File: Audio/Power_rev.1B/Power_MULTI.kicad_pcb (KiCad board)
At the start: 2 copper layers, 175.3 x 76.2 mm, 76 parts, among them P1 CONN_01X02, P2 CONN_01X02, P3 CONN_01X02, P4 CONN_01X02, Q1 NPN(TO-220-BCE), Q2 PNP(TO-220-BCE), Q3 NPN(TO-220-BCE), Q4 PNP(TO-220-BCE)

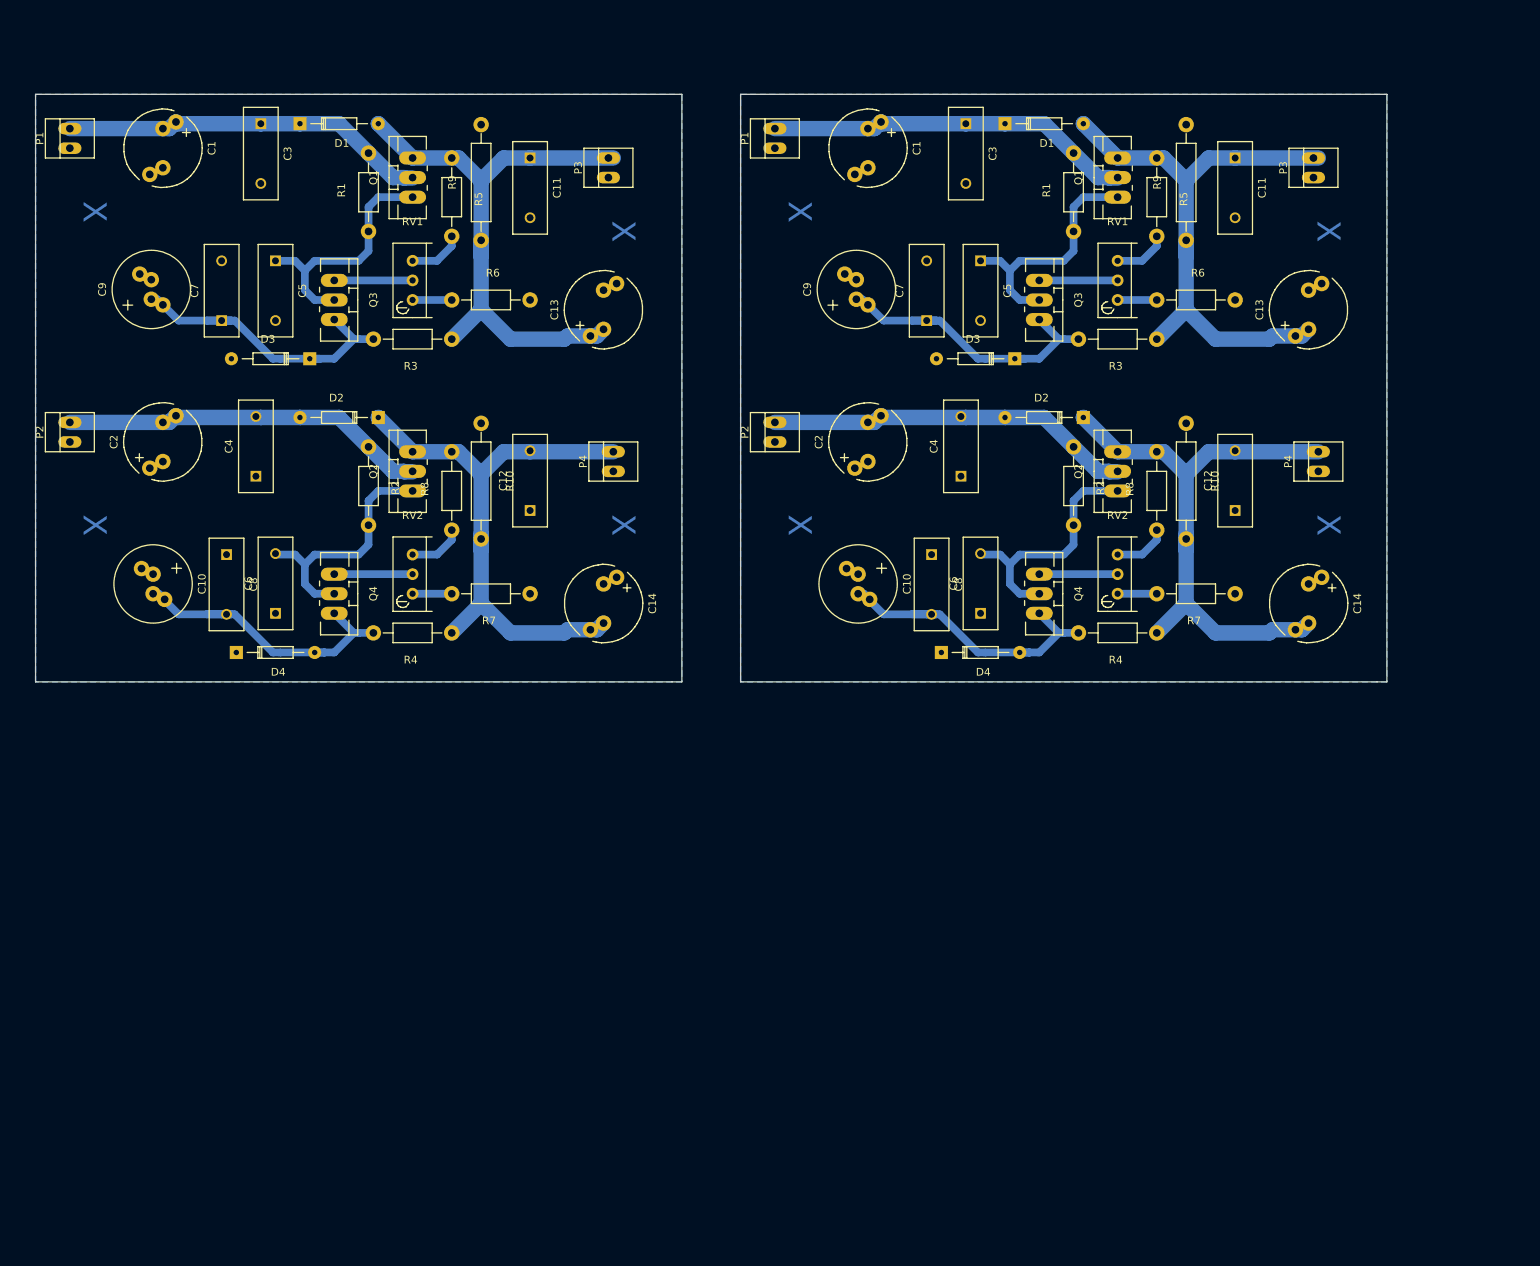
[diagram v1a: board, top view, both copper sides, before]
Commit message: Fixes
More fixes done
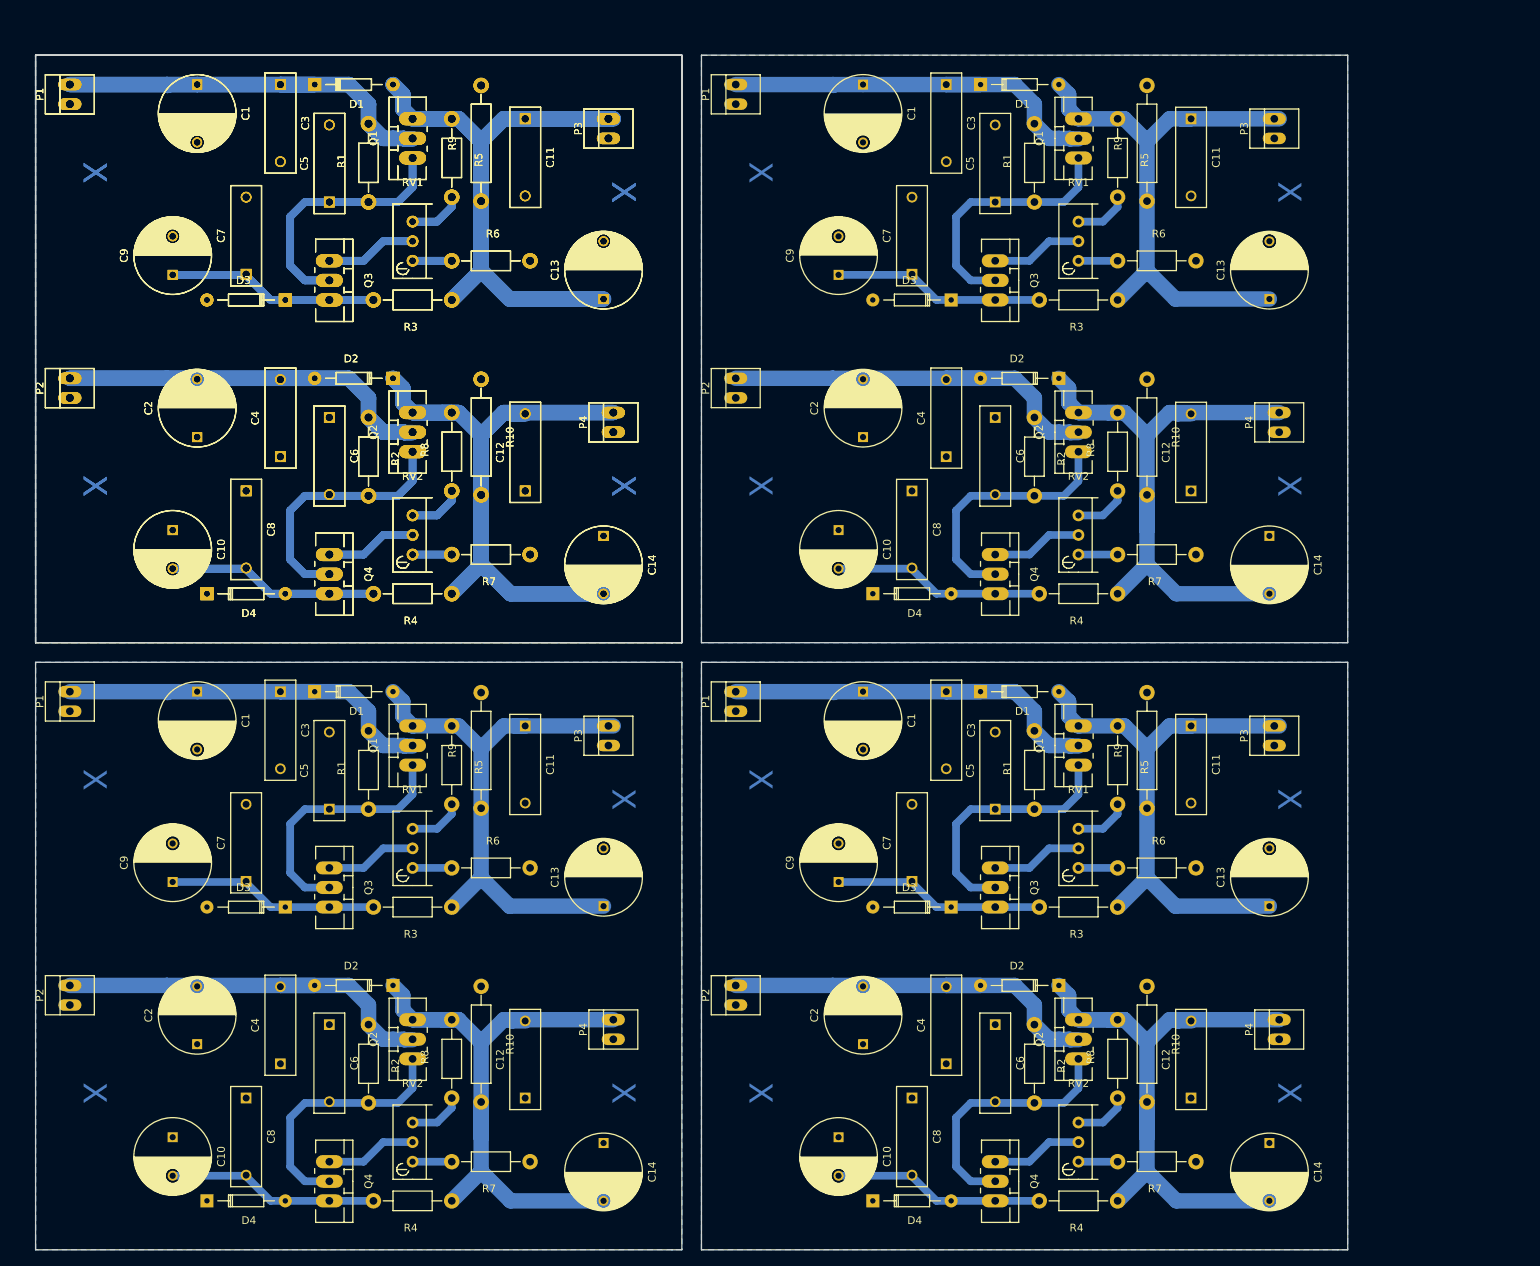
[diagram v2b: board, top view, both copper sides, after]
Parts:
- removed the C1 at (41.9, 37.5)
- removed the C1 at (133.3, 37.5)
- removed the C10 at (40.6, 94.0)
- removed the C10 at (132.1, 94.0)
- removed the C11 at (89.5, 38.7)
- removed the C11 at (181.0, 38.7)
- removed the C12 at (89.5, 84.5)
- removed the C12 at (181.0, 84.5)
- removed the C13 at (99.1, 58.4)
- removed the C13 at (190.5, 58.4)
- removed the C14 at (99.1, 96.5)
- removed the C14 at (190.5, 96.5)
- removed the C2 at (41.9, 75.6)
- removed the C2 at (133.3, 75.6)
- removed the C3 at (54.6, 34.3)
- removed the C3 at (146.1, 34.3)
- removed the C4 at (54.0, 80.0)
- removed the C4 at (145.4, 80.0)
- removed the C5 at (56.5, 52.1)
- removed the C5 at (148.0, 52.1)
- removed the C6 at (56.5, 97.8)
- removed the C6 at (148.0, 97.8)
- removed the C7 at (49.5, 59.8)
- removed the C7 at (141.0, 59.8)
- removed the C8 at (50.2, 90.2)
- removed the C8 at (141.6, 90.2)
- removed the C9 at (40.4, 55.8)
- removed the C9 at (131.8, 55.8)
- removed the D1 at (59.7, 34.3)
- removed the D1 at (151.1, 34.3)
- removed the D2 at (69.8, 72.4)
- removed the D2 at (161.3, 72.4)
- removed the D3 at (61.0, 64.8)
- removed the D3 at (152.4, 64.8)
- removed the D4 at (51.4, 102.9)
- removed the D4 at (142.9, 102.9)
- removed the P1 at (29.8, 36.2)
- removed the P1 at (121.3, 36.2)
- removed the P2 at (29.8, 74.3)
- removed the P2 at (121.3, 74.3)
- removed the P3 at (99.7, 40.0)
- removed the P3 at (191.1, 40.0)
- removed the P4 at (100.3, 78.1)
- removed the P4 at (191.8, 78.1)
- removed the Q1 at (74.3, 41.3)
- removed the Q1 at (165.7, 41.3)
- removed the Q2 at (74.3, 79.4)
- removed the Q2 at (165.7, 79.4)
- removed the Q3 at (64.1, 57.1)
- removed the Q3 at (155.6, 57.1)
- removed the Q4 at (64.1, 95.2)
- removed the Q4 at (155.6, 95.2)
- removed the R1 at (68.6, 43.2)
- removed the R1 at (160.0, 43.2)
- removed the R10 at (83.2, 80.6)
- removed the R10 at (174.6, 80.6)
- removed the R2 at (68.6, 81.3)
- removed the R2 at (160.0, 81.3)
- removed the R3 at (74.3, 62.2)
- removed the R3 at (165.7, 62.2)
- removed the R4 at (74.3, 100.3)
- removed the R4 at (165.7, 100.3)
- removed the R5 at (79.4, 43.8)
- removed the R5 at (170.8, 43.8)
- removed the R6 at (84.5, 57.1)
- removed the R6 at (175.9, 57.1)
- removed the R7 at (84.5, 95.2)
- removed the R7 at (175.9, 95.2)
- removed the R8 at (79.4, 81.9)
- removed the R8 at (170.8, 81.9)
- removed the R9 at (83.2, 41.9)
- removed the R9 at (174.6, 41.9)
- removed the RV1 at (74.3, 57.1)
- removed the RV1 at (165.7, 57.1)
- removed the RV2 at (74.3, 95.2)
- removed the RV2 at (165.7, 95.2)
- added C1 (x2): 820uF,100V, Capacitors_ThroughHole:C_Radial_D10_L20_P7.5, F.Cu at (46.4, 29.2)
- added C1: 820uF,100V, Capacitors_ThroughHole:C_Radial_D10_L20_P7.5, F.Cu at (46.4, 108.0)
- added C1: 820uF,100V, Capacitors_ThroughHole:C_Radial_D10_L20_P7.5, F.Cu at (132.7, 29.2)
- added C1: 820uF,100V, Capacitors_ThroughHole:C_Radial_D10_L20_P7.5, F.Cu at (132.7, 108.0)
- added C10 (x2): 22uF,60V+, Capacitors_ThroughHole:C_Radial_D10_L20_P5, F.Cu at (43.2, 87.0)
- added C10: 22uF,60V+, Capacitors_ThroughHole:C_Radial_D10_L20_P5, F.Cu at (43.2, 165.7)
- added C10: 22uF,60V+, Capacitors_ThroughHole:C_Radial_D10_L20_P5, F.Cu at (129.5, 87.0)
- added C10: 22uF,60V+, Capacitors_ThroughHole:C_Radial_D10_L20_P5, F.Cu at (129.5, 165.7)
- added C11 (x2): 0.1uF,60V+, Capacitors_ThroughHole:C_Rect_L13_W4_P10, F.Cu at (88.9, 33.7)
- added C11: 0.1uF,60V+, Capacitors_ThroughHole:C_Rect_L13_W4_P10, F.Cu at (88.9, 112.4)
- added C11: 0.1uF,60V+, Capacitors_ThroughHole:C_Rect_L13_W4_P10, F.Cu at (175.3, 33.7)
- added C11: 0.1uF,60V+, Capacitors_ThroughHole:C_Rect_L13_W4_P10, F.Cu at (175.3, 112.4)
- added C12 (x2): 0.1uF,60V+, Capacitors_ThroughHole:C_Rect_L13_W4_P10, F.Cu at (88.9, 81.9)
- added C12: 0.1uF,60V+, Capacitors_ThroughHole:C_Rect_L13_W4_P10, F.Cu at (88.9, 160.7)
- added C12: 0.1uF,60V+, Capacitors_ThroughHole:C_Rect_L13_W4_P10, F.Cu at (175.3, 81.9)
- added C12: 0.1uF,60V+, Capacitors_ThroughHole:C_Rect_L13_W4_P10, F.Cu at (175.3, 160.7)
- added C13 (x2): 470uF,200V, Capacitors_ThroughHole:C_Radial_D10_L20_P7.5, F.Cu at (99.1, 57.0)
- added C13: 470uF,200V, Capacitors_ThroughHole:C_Radial_D10_L20_P7.5, F.Cu at (99.1, 135.8)
- added C13: 470uF,200V, Capacitors_ThroughHole:C_Radial_D10_L20_P7.5, F.Cu at (185.4, 57.0)
- added C13: 470uF,200V, Capacitors_ThroughHole:C_Radial_D10_L20_P7.5, F.Cu at (185.4, 135.8)
- added C14 (x2): 470uF,200V, Capacitors_ThroughHole:C_Radial_D10_L20_P7.5, F.Cu at (99.1, 87.8)
- added C14: 470uF,200V, Capacitors_ThroughHole:C_Radial_D10_L20_P7.5, F.Cu at (99.1, 166.5)
- added C14: 470uF,200V, Capacitors_ThroughHole:C_Radial_D10_L20_P7.5, F.Cu at (185.4, 87.8)
- added C14: 470uF,200V, Capacitors_ThroughHole:C_Radial_D10_L20_P7.5, F.Cu at (185.4, 166.5)
- added C2 (x2): 820uF,100V, Capacitors_ThroughHole:C_Radial_D10_L20_P7.5, F.Cu at (46.4, 74.9)
- added C2: 820uF,100V, Capacitors_ThroughHole:C_Radial_D10_L20_P7.5, F.Cu at (46.4, 153.7)
- added C2: 820uF,100V, Capacitors_ThroughHole:C_Radial_D10_L20_P7.5, F.Cu at (132.7, 74.9)
- added C2: 820uF,100V, Capacitors_ThroughHole:C_Radial_D10_L20_P7.5, F.Cu at (132.7, 153.7)
- added C3 (x2): 0.1uF,125V, Capacitors_ThroughHole:C_Rect_L13_W4_P10, F.Cu at (57.1, 29.2)
- added C3: 0.1uF,125V, Capacitors_ThroughHole:C_Rect_L13_W4_P10, F.Cu at (57.1, 108.0)
- added C3: 0.1uF,125V, Capacitors_ThroughHole:C_Rect_L13_W4_P10, F.Cu at (143.5, 29.2)
- added C3: 0.1uF,125V, Capacitors_ThroughHole:C_Rect_L13_W4_P10, F.Cu at (143.5, 108.0)
- added C4 (x2): 0.1uF,125V, Capacitors_ThroughHole:C_Rect_L13_W4_P10, F.Cu at (57.1, 77.5)
- added C4: 0.1uF,125V, Capacitors_ThroughHole:C_Rect_L13_W4_P10, F.Cu at (57.1, 156.2)
- added C4: 0.1uF,125V, Capacitors_ThroughHole:C_Rect_L13_W4_P10, F.Cu at (143.5, 77.5)
- added C4: 0.1uF,125V, Capacitors_ThroughHole:C_Rect_L13_W4_P10, F.Cu at (143.5, 156.2)
- added C5 (x2): 0.47uF,125V, Capacitors_ThroughHole:C_Rect_L13_W4_P10, F.Cu at (63.5, 44.5)
- added C5: 0.47uF,125V, Capacitors_ThroughHole:C_Rect_L13_W4_P10, F.Cu at (63.5, 123.2)
- added C5: 0.47uF,125V, Capacitors_ThroughHole:C_Rect_L13_W4_P10, F.Cu at (149.9, 44.5)
- added C5: 0.47uF,125V, Capacitors_ThroughHole:C_Rect_L13_W4_P10, F.Cu at (149.9, 123.2)
- added C6 (x2): 0.47uF,125V, Capacitors_ThroughHole:C_Rect_L13_W4_P10, F.Cu at (63.5, 72.4)
- added C6: 0.47uF,125V, Capacitors_ThroughHole:C_Rect_L13_W4_P10, F.Cu at (63.5, 151.1)
- added C6: 0.47uF,125V, Capacitors_ThroughHole:C_Rect_L13_W4_P10, F.Cu at (149.9, 72.4)
- added C6: 0.47uF,125V, Capacitors_ThroughHole:C_Rect_L13_W4_P10, F.Cu at (149.9, 151.1)
- added C7 (x2): 0.1uF,60V+, Capacitors_ThroughHole:C_Rect_L13_W4_P10, F.Cu at (52.7, 53.8)
- added C7: 0.1uF,60V+, Capacitors_ThroughHole:C_Rect_L13_W4_P10, F.Cu at (52.7, 132.6)
- added C7: 0.1uF,60V+, Capacitors_ThroughHole:C_Rect_L13_W4_P10, F.Cu at (139.1, 53.8)
- added C7: 0.1uF,60V+, Capacitors_ThroughHole:C_Rect_L13_W4_P10, F.Cu at (139.1, 132.6)
- added C8 (x2): 0.1uF,60V+, Capacitors_ThroughHole:C_Rect_L13_W4_P10, F.Cu at (52.7, 81.9)
- added C8: 0.1uF,60V+, Capacitors_ThroughHole:C_Rect_L13_W4_P10, F.Cu at (52.7, 160.7)
- added C8: 0.1uF,60V+, Capacitors_ThroughHole:C_Rect_L13_W4_P10, F.Cu at (139.1, 81.9)
- added C8: 0.1uF,60V+, Capacitors_ThroughHole:C_Rect_L13_W4_P10, F.Cu at (139.1, 160.7)
- added C9 (x2): 22uF,60V+, Capacitors_ThroughHole:C_Radial_D10_L20_P5, F.Cu at (43.2, 53.9)
- added C9: 22uF,60V+, Capacitors_ThroughHole:C_Radial_D10_L20_P5, F.Cu at (43.2, 132.6)
- added C9: 22uF,60V+, Capacitors_ThroughHole:C_Radial_D10_L20_P5, F.Cu at (129.5, 53.9)
- added C9: 22uF,60V+, Capacitors_ThroughHole:C_Radial_D10_L20_P5, F.Cu at (129.5, 132.6)
- added D1 (x2): D, Diodes_ThroughHole:Diode_DO-35_SOD27_Horizontal_RM10, F.Cu at (61.6, 29.2)
- added D1: D, Diodes_ThroughHole:Diode_DO-35_SOD27_Horizontal_RM10, F.Cu at (61.6, 108.0)
- added D1: D, Diodes_ThroughHole:Diode_DO-35_SOD27_Horizontal_RM10, F.Cu at (148.0, 29.2)
- added D1: D, Diodes_ThroughHole:Diode_DO-35_SOD27_Horizontal_RM10, F.Cu at (148.0, 108.0)
- added D2 (x2): D, Diodes_ThroughHole:Diode_DO-35_SOD27_Horizontal_RM10, F.Cu at (71.8, 67.3)
- added D2: D, Diodes_ThroughHole:Diode_DO-35_SOD27_Horizontal_RM10, F.Cu at (71.8, 146.1)
- added D2: D, Diodes_ThroughHole:Diode_DO-35_SOD27_Horizontal_RM10, F.Cu at (158.1, 67.3)
- added D2: D, Diodes_ThroughHole:Diode_DO-35_SOD27_Horizontal_RM10, F.Cu at (158.1, 146.1)
- added D3 (x2): ZENER, Diodes_ThroughHole:Diode_DO-35_SOD27_Horizontal_RM10, F.Cu at (57.8, 57.1)
- added D3: ZENER, Diodes_ThroughHole:Diode_DO-35_SOD27_Horizontal_RM10, F.Cu at (57.8, 135.9)
- added D3: ZENER, Diodes_ThroughHole:Diode_DO-35_SOD27_Horizontal_RM10, F.Cu at (144.1, 57.1)
- added D3: ZENER, Diodes_ThroughHole:Diode_DO-35_SOD27_Horizontal_RM10, F.Cu at (144.1, 135.9)
- added D4 (x2): ZENER, Diodes_ThroughHole:Diode_DO-35_SOD27_Horizontal_RM10, F.Cu at (47.6, 95.2)
- added D4: ZENER, Diodes_ThroughHole:Diode_DO-35_SOD27_Horizontal_RM10, F.Cu at (47.6, 174.0)
- added D4: ZENER, Diodes_ThroughHole:Diode_DO-35_SOD27_Horizontal_RM10, F.Cu at (134.0, 95.2)
- added D4: ZENER, Diodes_ThroughHole:Diode_DO-35_SOD27_Horizontal_RM10, F.Cu at (134.0, 174.0)
- added P1 (x2): CONN_01X02, Connect:PINHEAD1-2, F.Cu at (29.8, 30.5)
- added P1: CONN_01X02, Connect:PINHEAD1-2, F.Cu at (29.8, 109.2)
- added P1: CONN_01X02, Connect:PINHEAD1-2, F.Cu at (116.2, 30.5)
- added P1: CONN_01X02, Connect:PINHEAD1-2, F.Cu at (116.2, 109.2)
- added P2 (x2): CONN_01X02, Connect:PINHEAD1-2, F.Cu at (29.8, 68.6)
- added P2: CONN_01X02, Connect:PINHEAD1-2, F.Cu at (29.8, 147.3)
- added P2: CONN_01X02, Connect:PINHEAD1-2, F.Cu at (116.2, 68.6)
- added P2: CONN_01X02, Connect:PINHEAD1-2, F.Cu at (116.2, 147.3)
- added P3 (x2): CONN_01X02, Connect:PINHEAD1-2, F.Cu at (99.7, 34.9)
- added P3: CONN_01X02, Connect:PINHEAD1-2, F.Cu at (99.7, 113.7)
- added P3: CONN_01X02, Connect:PINHEAD1-2, F.Cu at (186.1, 34.9)
- added P3: CONN_01X02, Connect:PINHEAD1-2, F.Cu at (186.1, 113.7)
- added P4 (x2): CONN_01X02, Connect:PINHEAD1-2, F.Cu at (100.3, 73.0)
- added P4: CONN_01X02, Connect:PINHEAD1-2, F.Cu at (100.3, 151.8)
- added P4: CONN_01X02, Connect:PINHEAD1-2, F.Cu at (186.7, 73.0)
- added P4: CONN_01X02, Connect:PINHEAD1-2, F.Cu at (186.7, 151.8)
- added Q1 (x2): NPN(TO-220-BCE), TO_SOT_Packages_THT:TO-220_Neutral123_Vertical_LargePads, F.Cu at (74.3, 36.2)
- added Q1: NPN(TO-220-BCE), TO_SOT_Packages_THT:TO-220_Neutral123_Vertical_LargePads, F.Cu at (74.3, 114.9)
- added Q1: NPN(TO-220-BCE), TO_SOT_Packages_THT:TO-220_Neutral123_Vertical_LargePads, F.Cu at (160.7, 36.2)
- added Q1: NPN(TO-220-BCE), TO_SOT_Packages_THT:TO-220_Neutral123_Vertical_LargePads, F.Cu at (160.7, 114.9)
- added Q2 (x2): PNP(TO-220-BCE), TO_SOT_Packages_THT:TO-220_Neutral123_Vertical_LargePads, F.Cu at (74.3, 74.3)
- added Q2: PNP(TO-220-BCE), TO_SOT_Packages_THT:TO-220_Neutral123_Vertical_LargePads, F.Cu at (74.3, 153.0)
- added Q2: PNP(TO-220-BCE), TO_SOT_Packages_THT:TO-220_Neutral123_Vertical_LargePads, F.Cu at (160.7, 74.3)
- added Q2: PNP(TO-220-BCE), TO_SOT_Packages_THT:TO-220_Neutral123_Vertical_LargePads, F.Cu at (160.7, 153.0)
- added Q3 (x2): NPN(TO-220-BCE), TO_SOT_Packages_THT:TO-220_Neutral123_Vertical_LargePads, F.Cu at (63.5, 54.6)
- added Q3: NPN(TO-220-BCE), TO_SOT_Packages_THT:TO-220_Neutral123_Vertical_LargePads, F.Cu at (63.5, 133.3)
- added Q3: NPN(TO-220-BCE), TO_SOT_Packages_THT:TO-220_Neutral123_Vertical_LargePads, F.Cu at (149.9, 54.6)
- added Q3: NPN(TO-220-BCE), TO_SOT_Packages_THT:TO-220_Neutral123_Vertical_LargePads, F.Cu at (149.9, 133.3)
- added Q4 (x2): PNP(TO-220-BCE), TO_SOT_Packages_THT:TO-220_Neutral123_Vertical_LargePads, F.Cu at (63.5, 92.7)
- added Q4: PNP(TO-220-BCE), TO_SOT_Packages_THT:TO-220_Neutral123_Vertical_LargePads, F.Cu at (63.5, 171.4)
- added Q4: PNP(TO-220-BCE), TO_SOT_Packages_THT:TO-220_Neutral123_Vertical_LargePads, F.Cu at (149.9, 92.7)
- added Q4: PNP(TO-220-BCE), TO_SOT_Packages_THT:TO-220_Neutral123_Vertical_LargePads, F.Cu at (149.9, 171.4)
- added R1 (x2): 18k, Resistors_ThroughHole:Resistor_Horizontal_RM10mm, F.Cu at (68.6, 39.4)
- added R1: 18k, Resistors_ThroughHole:Resistor_Horizontal_RM10mm, F.Cu at (68.6, 118.1)
- added R1: 18k, Resistors_ThroughHole:Resistor_Horizontal_RM10mm, F.Cu at (154.9, 39.4)
- added R1: 18k, Resistors_ThroughHole:Resistor_Horizontal_RM10mm, F.Cu at (154.9, 118.1)
- added R10 (x2): 8.2k,0.5W+, Resistors_ThroughHole:Resistor_Horizontal_RM15mm, F.Cu at (83.2, 74.9)
- added R10: 8.2k,0.5W+, Resistors_ThroughHole:Resistor_Horizontal_RM15mm, F.Cu at (83.2, 153.7)
- added R10: 8.2k,0.5W+, Resistors_ThroughHole:Resistor_Horizontal_RM15mm, F.Cu at (169.5, 74.9)
- added R10: 8.2k,0.5W+, Resistors_ThroughHole:Resistor_Horizontal_RM15mm, F.Cu at (169.5, 153.7)
- added R2 (x2): 18k, Resistors_ThroughHole:Resistor_Horizontal_RM10mm, F.Cu at (68.6, 77.5)
- added R2: 18k, Resistors_ThroughHole:Resistor_Horizontal_RM10mm, F.Cu at (68.6, 156.2)
- added R2: 18k, Resistors_ThroughHole:Resistor_Horizontal_RM10mm, F.Cu at (154.9, 77.5)
- added R2: 18k, Resistors_ThroughHole:Resistor_Horizontal_RM10mm, F.Cu at (154.9, 156.2)
- added R3 (x2): 4.3k, Resistors_ThroughHole:Resistor_Horizontal_RM10mm, F.Cu at (74.3, 57.1)
- added R3: 4.3k, Resistors_ThroughHole:Resistor_Horizontal_RM10mm, F.Cu at (74.3, 135.9)
- added R3: 4.3k, Resistors_ThroughHole:Resistor_Horizontal_RM10mm, F.Cu at (160.7, 57.1)
- added R3: 4.3k, Resistors_ThroughHole:Resistor_Horizontal_RM10mm, F.Cu at (160.7, 135.9)
- added R4 (x2): 4.3k, Resistors_ThroughHole:Resistor_Horizontal_RM10mm, F.Cu at (74.3, 95.2)
- added R4: 4.3k, Resistors_ThroughHole:Resistor_Horizontal_RM10mm, F.Cu at (74.3, 174.0)
- added R4: 4.3k, Resistors_ThroughHole:Resistor_Horizontal_RM10mm, F.Cu at (160.7, 95.2)
- added R4: 4.3k, Resistors_ThroughHole:Resistor_Horizontal_RM10mm, F.Cu at (160.7, 174.0)
- added R5 (x2): 20k, Resistors_ThroughHole:Resistor_Horizontal_RM10mm, F.Cu at (79.4, 38.7)
- added R5: 20k, Resistors_ThroughHole:Resistor_Horizontal_RM10mm, F.Cu at (79.4, 117.5)
- added R5: 20k, Resistors_ThroughHole:Resistor_Horizontal_RM10mm, F.Cu at (165.7, 38.7)
- added R5: 20k, Resistors_ThroughHole:Resistor_Horizontal_RM10mm, F.Cu at (165.7, 117.5)
- added R6 (x2): 27k, Resistors_ThroughHole:Resistor_Horizontal_RM10mm, F.Cu at (84.5, 52.1)
- added R6: 27k, Resistors_ThroughHole:Resistor_Horizontal_RM10mm, F.Cu at (84.5, 130.8)
- added R6: 27k, Resistors_ThroughHole:Resistor_Horizontal_RM10mm, F.Cu at (170.8, 52.1)
- added R6: 27k, Resistors_ThroughHole:Resistor_Horizontal_RM10mm, F.Cu at (170.8, 130.8)
- added R7 (x2): 27k, Resistors_ThroughHole:Resistor_Horizontal_RM10mm, F.Cu at (84.5, 90.2)
- added R7: 27k, Resistors_ThroughHole:Resistor_Horizontal_RM10mm, F.Cu at (84.5, 168.9)
- added R7: 27k, Resistors_ThroughHole:Resistor_Horizontal_RM10mm, F.Cu at (170.8, 90.2)
- added R7: 27k, Resistors_ThroughHole:Resistor_Horizontal_RM10mm, F.Cu at (170.8, 168.9)
- added R8 (x2): 20k, Resistors_ThroughHole:Resistor_Horizontal_RM10mm, F.Cu at (79.4, 76.8)
- added R8: 20k, Resistors_ThroughHole:Resistor_Horizontal_RM10mm, F.Cu at (79.4, 155.6)
- added R8: 20k, Resistors_ThroughHole:Resistor_Horizontal_RM10mm, F.Cu at (165.7, 76.8)
- added R8: 20k, Resistors_ThroughHole:Resistor_Horizontal_RM10mm, F.Cu at (165.7, 155.6)
- added R9 (x2): 8.2k,0.5W+, Resistors_ThroughHole:Resistor_Horizontal_RM15mm, F.Cu at (83.2, 36.8)
- added R9: 8.2k,0.5W+, Resistors_ThroughHole:Resistor_Horizontal_RM15mm, F.Cu at (83.2, 115.6)
- added R9: 8.2k,0.5W+, Resistors_ThroughHole:Resistor_Horizontal_RM15mm, F.Cu at (169.5, 36.8)
- added R9: 8.2k,0.5W+, Resistors_ThroughHole:Resistor_Horizontal_RM15mm, F.Cu at (169.5, 115.6)
- added RV1 (x2): 10k, Potentiometers:Potentiometer_Bourns_3296W_3-8Zoll_Inline_ScrewUp, F.Cu at (74.3, 52.1)
- added RV1: 10k, Potentiometers:Potentiometer_Bourns_3296W_3-8Zoll_Inline_ScrewUp, F.Cu at (74.3, 130.8)
- added RV1: 10k, Potentiometers:Potentiometer_Bourns_3296W_3-8Zoll_Inline_ScrewUp, F.Cu at (160.7, 52.1)
- added RV1: 10k, Potentiometers:Potentiometer_Bourns_3296W_3-8Zoll_Inline_ScrewUp, F.Cu at (160.7, 130.8)
- added RV2 (x2): 10k, Potentiometers:Potentiometer_Bourns_3296W_3-8Zoll_Inline_ScrewUp, F.Cu at (74.3, 90.2)
- added RV2: 10k, Potentiometers:Potentiometer_Bourns_3296W_3-8Zoll_Inline_ScrewUp, F.Cu at (74.3, 168.9)
- added RV2: 10k, Potentiometers:Potentiometer_Bourns_3296W_3-8Zoll_Inline_ScrewUp, F.Cu at (160.7, 90.2)
- added RV2: 10k, Potentiometers:Potentiometer_Bourns_3296W_3-8Zoll_Inline_ScrewUp, F.Cu at (160.7, 168.9)
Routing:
- net VEE: track 153.9 -> 447.1 mm
- net VCC: track 153.9 -> 374.2 mm
- net 63-75V(-): track 95.6 -> 267.4 mm
- net 63-75V(+): track 95.6 -> 267.4 mm
- net Net-(C6-Pad2): track 65.0 -> 167.4 mm
- net Net-(C5-Pad1): track 65.0 -> 167.4 mm
- net Net-(C10-Pad2): track 84.7 -> 137.7 mm
- net Net-(C7-Pad1): track 84.7 -> 137.7 mm
- net Net-(Q4-Pad1): track 20.3 -> 59.2 mm
- net Net-(Q3-Pad1): track 20.3 -> 59.2 mm
- net Net-(R8-Pad1): track 14.3 -> 35.7 mm
- net Net-(R5-Pad2): track 14.3 -> 35.7 mm
- net Net-(R7-Pad2): track 10.2 -> 25.4 mm
- net Net-(R6-Pad1): track 10.2 -> 25.4 mm
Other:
- board size 175.3 x 76.2 mm -> 170.2 x 154.9 mm
